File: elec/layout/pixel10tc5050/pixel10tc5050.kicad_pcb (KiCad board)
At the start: 2 copper layers, 2 parts

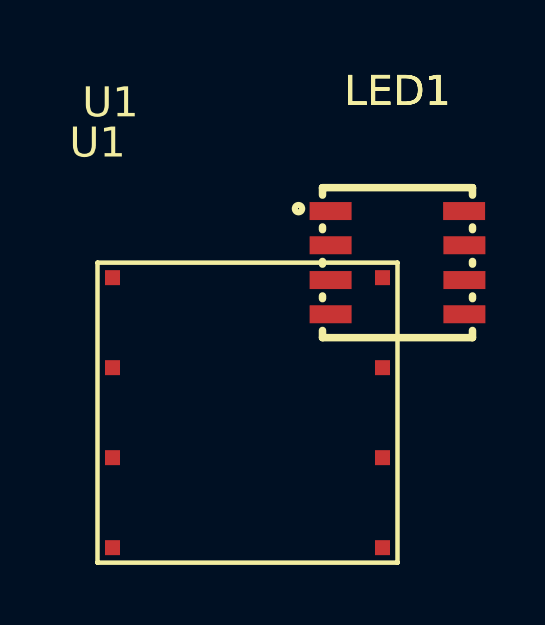
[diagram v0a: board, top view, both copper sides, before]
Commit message: updating rp2040
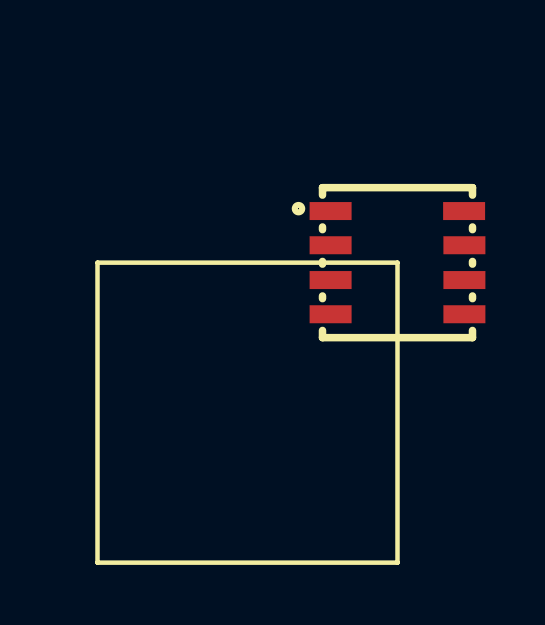
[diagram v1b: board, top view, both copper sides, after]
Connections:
- LED1 pad 5: cathode_cold_white -> rgb-cathodes-cathode-1
- LED1 pad 6: cathode_blue -> rgb-cathodes-cathode-0
- LED1 pad 7: cathode_green -> rgb-cathodes-cathode-2
- LED1 pad 8: cathode_red -> rgb-cathodes-cathode-3
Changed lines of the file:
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@@
     )
     (net 0 "")
-    (net 1 "cathode_blue")
-    (net 2 "cathode_cold_white")
-    (net 3 "cathode_green")
-    (net 4 "cathode_red")
-    (net 5 "cathode_uv")
+    (net 1 "rgb-cathodes-cathode-0")
+    (net 2 "rgb-cathodes-cathode-1")
+    (net 3 "rgb-cathodes-cathode-2")
+    (net 4 "rgb-cathodes-cathode-3")
     (net 6 "anode")
-    (net 7 "cathode_ir")
-    (net 8 "cathode_warm_white")
     (footprint "ATOPILE_PIXEL10:pixel10"
         (layer "F.Cu")
@@
             (at 0.43 -5.34 0)
             (layer "F.SilkS")
-            (hide no)
+            (hide yes)
             (effects
                 (font
@@
             )
         )
-        (property "__atopile_lib_fp_hash__" "28afaa8a-933c-de95-36da-41610e57d330"
+        (property "__atopile_lib_fp_hash__" "b5aa9518-1f07-5a56-08b4-48067117c1be"
             (at 0 0 0)
             (layer "User.9")
@@
         )
         (attr smd)
+        (fp_line
+            (start 0 0)
+            (end 0 10)
+            (stroke
+                (width 0.15)
+                (type solid)
+            )
+            (layer "F.SilkS")
+        )
         (fp_line
             (start 0 0)
@@
             (start 0 10)
             (end 10 10)
-            (stroke
-                (width 0.15)
-                (type solid)
-            )
-            (layer "F.SilkS")
-        )
-        (fp_line
-            (start 0 0)
-            (end 0 10)
             (stroke
                 (width 0.15)
@@
                     (thickness 0.15)
                 )
+                (hide yes)
             )
             (unlocked no)
@@
                     (thickness 0.15)
                 )
+                (hide yes)
             )
             (unlocked no)
-        )
-        (pad "1" smd rect
-            (at 0.5 0.5 0)
-            (size 0.5 0.5)
-            (layers "F.Cu" "F.Mask" "F.Paste")
-            (net 6 "anode")
-        )
-        (pad "2" smd rect
-            (at 0.5 3.5 0)
-            (size 0.5 0.5)
-            (layers "F.Cu" "F.Mask" "F.Paste")
-            (net 4 "cathode_red")
-        )
-        (pad "3" smd rect
-            (at 0.5 6.5 0)
-            (size 0.5 0.5)
-            (layers "F.Cu" "F.Mask" "F.Paste")
-            (net 3 "cathode_green")
-        )
-        (pad "4" smd rect
-            (at 0.5 9.5 0)
-            (size 0.5 0.5)
-            (layers "F.Cu" "F.Mask" "F.Paste")
-            (net 1 "cathode_blue")
-        )
-        (pad "5" smd rect
-            (at 9.5 0.5 0)
-            (size 0.5 0.5)
-            (layers "F.Cu" "F.Mask" "F.Paste")
-            (net 8 "cathode_warm_white")
-        )
-        (pad "6" smd rect
-            (at 9.5 3.5 0)
-            (size 0.5 0.5)
-            (layers "F.Cu" "F.Mask" "F.Paste")
-            (net 2 "cathode_cold_white")
-        )
-        (pad "7" smd rect
-            (at 9.5 6.5 0)
-            (size 0.5 0.5)
-            (layers "F.Cu" "F.Mask" "F.Paste")
-            (net 5 "cathode_uv")
-        )
-        (pad "8" smd rect
-            (at 9.5 9.5 0)
-            (size 0.5 0.5)
-            (layers "F.Cu" "F.Mask" "F.Paste")
-            (net 7 "cathode_ir")
         )
         (embedded_fonts no)
@@
             (at 0 -5.72 0)
             (layer "F.SilkS")
-            (hide no)
+            (hide yes)
             (effects
                 (font
@@
                     (thickness 0.15)
                 )
+                (hide yes)
             )
             (unlocked no)
@@
             (size 0.6 1.4)
             (layers "F.Cu" "F.Mask" "F.Paste")
-            (net 2 "cathode_cold_white")
+            (net 2 "rgb-cathodes-cathode-1")
         )
         (pad "6" smd rect
@@
             (size 0.6 1.4)
             (layers "F.Cu" "F.Mask" "F.Paste")
-            (net 1 "cathode_blue")
+            (net 1 "rgb-cathodes-cathode-0")
         )
         (pad "7" smd rect
@@
             (size 0.6 1.4)
             (layers "F.Cu" "F.Mask" "F.Paste")
-            (net 3 "cathode_green")
+            (net 3 "rgb-cathodes-cathode-2")
         )
         (pad "8" smd rect
@@
             (size 0.6 1.4)
             (layers "F.Cu" "F.Mask" "F.Paste")
-            (net 4 "cathode_red")
+            (net 4 "rgb-cathodes-cathode-3")
         )
         (model "${KIPRJMOD}/../../src/parts/TCWIN_TC5050RGBW4D06_4CJHR3_AFW421A/LED-SMD_8P-L5.0-W5.0-TL-FD.STEP"
